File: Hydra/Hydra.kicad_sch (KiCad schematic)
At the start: 116 parts, among them J1 USB_C_Receptacle_USB2.0, SW1 SW_Push, U1 USBLC6-2SC6, U2 ATmega32U4-M, Y1 16MHz

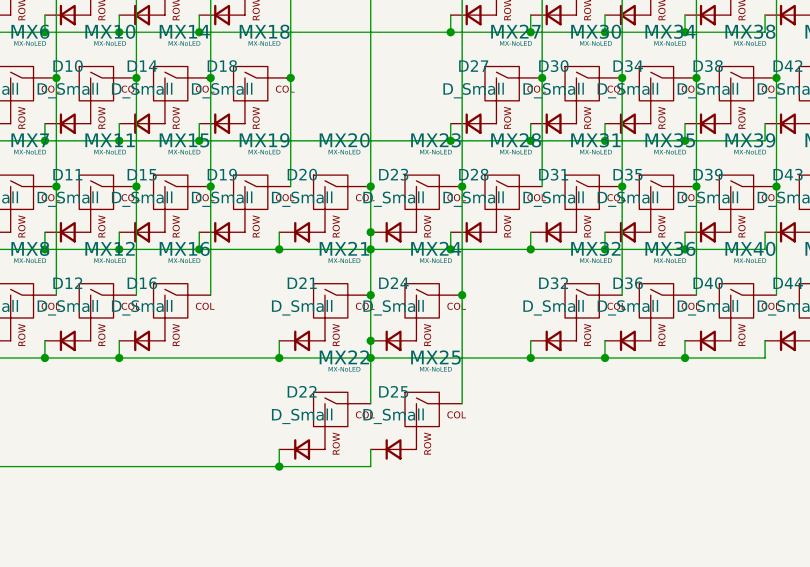
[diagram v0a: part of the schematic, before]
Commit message: Fixed Schematic
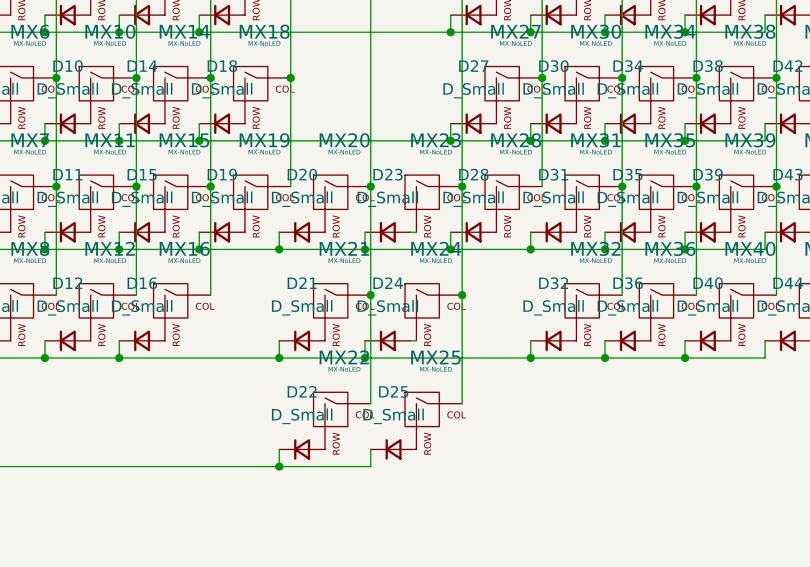
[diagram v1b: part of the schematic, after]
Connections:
- net COL5: no longer D11.1 (K), D12.1 (K), D15.1 (K), D16.1 (K), D19.1 (K), D20.1 (K), D21.1 (K), D23.1 (K), D24.1 (K), D28.1 (K), D3.1 (K), D31.1 (K), D32.1 (K), D35.1 (K), D36.1 (K), D39.1 (K), D4.1 (K), D40.1 (K), D43.1 (K), D44.1 (K), D7.1 (K), D8.1 (K)
- new net ROW2: D11.1 (K), D15.1 (K), D19.1 (K), D20.1 (K), D23.1 (K), D28.1 (K), D3.1 (K), D31.1 (K), D35.1 (K), D39.1 (K), D43.1 (K), D7.1 (K)
- new net ROW3: D12.1 (K), D16.1 (K), D21.1 (K), D24.1 (K), D32.1 (K), D36.1 (K), D4.1 (K), D40.1 (K), D44.1 (K), D8.1 (K)
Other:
- moved on the sheet: D23, D24
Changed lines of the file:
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@@
   (junction (at 68.58 111.125) (diameter 0) (color 0 0 0 0)
   )
-  (junction (at 91.44 64.135) (diameter 0) (color 0 0 0 0)
-  )
   (junction (at 191.135 41.275) (diameter 0) (color 0 0 0 0)
   )
@@
   (junction (at 117.475 52.07) (diameter 0) (color 0 0 0 0)
   )
+  (junction (at 91.44 57.15) (diameter 0) (color 0 0 0 0)
+  )
   (junction (at 144.145 142.24) (diameter 0) (color 0 0 0 0)
   )
+  (junction (at 91.44 69.215) (diameter 0) (color 0 0 0 0)
+  )
   (junction (at 46.355 40.005) (diameter 0) (color 0 0 0 0)
   )
-  (junction (at 91.44 69.215) (diameter 0) (color 0 0 0 0)
-  )
   (junction (at 82.55 45.085) (diameter 0) (color 0 0 0 0)
   )
@@
   (junction (at 55.245 40.005) (diameter 0) (color 0 0 0 0)
   )
-  (junction (at 91.44 57.15) (diameter 0) (color 0 0 0 0)
-  )
   (junction (at 109.22 64.135) (diameter 0) (color 0 0 0 0)
   )
@@
   (junction (at 217.805 31.115) (diameter 0) (color 0 0 0 0)
   )
-  (junction (at 91.44 74.295) (diameter 0) (color 0 0 0 0)
+  (junction (at 90.805 76.2) (diameter 0) (color 0 0 0 0)
   )
   (junction (at 81.28 76.2) (diameter 0) (color 0 0 0 0)
@@
   (junction (at 101.6 57.15) (diameter 0) (color 0 0 0 0)
   )
-  (junction (at 91.44 62.23) (diameter 0) (color 0 0 0 0)
-  )
   (junction (at 126.365 64.135) (diameter 0) (color 0 0 0 0)
   )
-  (junction (at 91.44 76.2) (diameter 0) (color 0 0 0 0)
-  )
   (junction (at 65.405 45.085) (diameter 0) (color 0 0 0 0)
   )
@@
   )
   (junction (at 63.5 52.07) (diameter 0) (color 0 0 0 0)
+  )
+  (junction (at 90.805 64.135) (diameter 0) (color 0 0 0 0)
   )
   (junction (at 55.245 64.135) (diameter 0) (color 0 0 0 0)
@@
     (stroke (width 0) (type default) (color 0 0 0 0))
   )
-  (wire (pts (xy 91.44 74.295) (xy 91.44 76.2))
+  (wire (pts (xy 91.44 69.215) (xy 91.44 81.28))
     (stroke (width 0) (type default) (color 0 0 0 0))
   )
@@
     (stroke (width 0) (type default) (color 0 0 0 0))
   )
-  (wire (pts (xy 91.44 62.23) (xy 91.44 64.135))
-    (stroke (width 0) (type default) (color 0 0 0 0))
-  )
   (wire (pts (xy 123.825 142.24) (xy 137.16 142.24))
     (stroke (width 0) (type default) (color 0 0 0 0))
@@
     (stroke (width 0) (type default) (color 0 0 0 0))
   )
-  (wire (pts (xy 91.44 76.2) (xy 81.28 76.2))
-    (stroke (width 0) (type default) (color 0 0 0 0))
-  )
   (wire (pts (xy 60.325 113.665) (xy 63.5 113.665))
     (stroke (width 0) (type default) (color 0 0 0 0))
@@
     (stroke (width 0) (type default) (color 0 0 0 0))
   )
+  (wire (pts (xy 91.44 57.15) (xy 91.44 69.215))
+    (stroke (width 0) (type default) (color 0 0 0 0))
+  )
   (wire (pts (xy 82.55 45.085) (xy 82.55 57.15))
     (stroke (width 0) (type default) (color 0 0 0 0))
@@
     (stroke (width 0) (type default) (color 0 0 0 0))
   )
+  (wire (pts (xy 90.805 62.23) (xy 90.805 64.135))
+    (stroke (width 0) (type default) (color 0 0 0 0))
+  )
   (wire (pts (xy 37.465 50.165) (xy 37.465 52.07))
     (stroke (width 0) (type default) (color 0 0 0 0))
@@
     (stroke (width 0) (type default) (color 0 0 0 0))
   )
-  (wire (pts (xy 91.44 57.15) (xy 91.44 62.23))
-    (stroke (width 0) (type default) (color 0 0 0 0))
-  )
   (wire (pts (xy 101.6 22.86) (xy 101.6 57.15))
     (stroke (width 0) (type default) (color 0 0 0 0))
@@
     (stroke (width 0) (type default) (color 0 0 0 0))
   )
+  (wire (pts (xy 95.885 62.23) (xy 96.52 62.23))
+    (stroke (width 0) (type default) (color 0 0 0 0))
+  )
   (wire (pts (xy 37.465 52.07) (xy 36.83 52.07))
     (stroke (width 0) (type default) (color 0 0 0 0))
   )
-  (wire (pts (xy 109.22 76.2) (xy 91.44 76.2))
+  (wire (pts (xy 81.28 76.2) (xy 90.805 76.2))
     (stroke (width 0) (type default) (color 0 0 0 0))
   )
@@
     (stroke (width 0) (type default) (color 0 0 0 0))
   )
-  (wire (pts (xy 91.44 76.2) (xy 91.44 81.28))
-    (stroke (width 0) (type default) (color 0 0 0 0))
-  )
   (wire (pts (xy 144.145 137.16) (xy 150.495 137.16))
     (stroke (width 0) (type default) (color 0 0 0 0))
@@
     (stroke (width 0) (type default) (color 0 0 0 0))
   )
+  (wire (pts (xy 90.805 76.2) (xy 109.22 76.2))
+    (stroke (width 0) (type default) (color 0 0 0 0))
+  )
   (wire (pts (xy 65.405 45.085) (xy 65.405 57.15))
     (stroke (width 0) (type default) (color 0 0 0 0))
@@
     (stroke (width 0) (type default) (color 0 0 0 0))
   )
-  (wire (pts (xy 91.44 64.135) (xy 81.28 64.135))
-    (stroke (width 0) (type default) (color 0 0 0 0))
-  )
   (wire (pts (xy 252.095 84.455) (xy 256.54 84.455))
     (stroke (width 0) (type default) (color 0 0 0 0))
@@
     (stroke (width 0) (type default) (color 0 0 0 0))
   )
+  (wire (pts (xy 95.885 74.295) (xy 96.52 74.295))
+    (stroke (width 0) (type default) (color 0 0 0 0))
+  )
   (wire (pts (xy 127.635 45.085) (xy 127.635 57.15))
     (stroke (width 0) (type default) (color 0 0 0 0))
@@
     (stroke (width 0) (type default) (color 0 0 0 0))
   )
-  (wire (pts (xy 100.33 64.135) (xy 91.44 64.135))
+  (wire (pts (xy 81.28 64.135) (xy 90.805 64.135))
     (stroke (width 0) (type default) (color 0 0 0 0))
   )
@@
     (stroke (width 0) (type default) (color 0 0 0 0))
   )
-  (wire (pts (xy 91.44 69.215) (xy 91.44 74.295))
-    (stroke (width 0) (type default) (color 0 0 0 0))
-  )
   (wire (pts (xy 36.83 76.2) (xy 36.83 74.295))
     (stroke (width 0) (type default) (color 0 0 0 0))
@@
     (stroke (width 0) (type default) (color 0 0 0 0))
   )
+  (wire (pts (xy 90.805 64.135) (xy 100.33 64.135))
+    (stroke (width 0) (type default) (color 0 0 0 0))
+  )
   (wire (pts (xy 203.2 31.115) (xy 205.74 31.115))
     (stroke (width 0) (type default) (color 0 0 0 0))
@@
     (stroke (width 0) (type default) (color 0 0 0 0))
   )
+  (wire (pts (xy 90.805 74.295) (xy 90.805 76.2))
+    (stroke (width 0) (type default) (color 0 0 0 0))
+  )
   (wire (pts (xy 100.33 38.1) (xy 100.33 40.005))
     (stroke (width 0) (type default) (color 0 0 0 0))
@@
   )
   (wire (pts (xy 135.255 64.135) (xy 126.365 64.135))
-    (stroke (width 0) (type default) (color 0 0 0 0))
-  )
-  (wire (pts (xy 91.44 64.135) (xy 91.44 69.215))
     (stroke (width 0) (type default) (color 0 0 0 0))
   )
@@
     (pin "1")
   )
-  (symbol (lib_id "Device:D_Small") (at 93.98 62.23 0) (unit 1)
-    (in_bom yes) (on_board yes) (fields_autoplaced)
-    (property "Reference" "D23" (id 0) (at 93.98 55.88 0))
-    (property "Value" "D_Small" (id 1) (at 93.98 58.42 0))
-    (property "Footprint" "Diode_SMD:D_SOD-123" (id 2) (at 93.98 62.23 90)
-      (effects (font (size 1.27 1.27)) hide)
-    )
-    (property "Datasheet" "~" (id 3) (at 93.98 62.23 90)
+  (symbol (lib_id "Device:D_Small") (at 93.345 62.23 0) (unit 1)
+    (in_bom yes) (on_board yes) (fields_autoplaced)
+    (property "Reference" "D23" (id 0) (at 93.345 55.88 0))
+    (property "Value" "D_Small" (id 1) (at 93.345 58.42 0))
+    (property "Footprint" "Diode_SMD:D_SOD-123" (id 2) (at 93.345 62.23 90)
+      (effects (font (size 1.27 1.27)) hide)
+    )
+    (property "Datasheet" "~" (id 3) (at 93.345 62.23 90)
       (effects (font (size 1.27 1.27)) hide)
     )
@@
     (pin "1")
   )
-  (symbol (lib_id "Device:D_Small") (at 93.98 74.295 0) (unit 1)
-    (in_bom yes) (on_board yes) (fields_autoplaced)
-    (property "Reference" "D24" (id 0) (at 93.98 67.945 0))
-    (property "Value" "D_Small" (id 1) (at 93.98 70.485 0))
-    (property "Footprint" "Diode_SMD:D_SOD-123" (id 2) (at 93.98 74.295 90)
-      (effects (font (size 1.27 1.27)) hide)
-    )
-    (property "Datasheet" "~" (id 3) (at 93.98 74.295 90)
-      (effects (font (size 1.27 1.27)) hide)
-    )
+  (symbol (lib_id "Device:D_Small") (at 93.345 74.295 0) (unit 1)
+    (in_bom yes) (on_board yes) (fields_autoplaced)
+    (property "Reference" "D24" (id 0) (at 93.345 67.945 0))
+    (property "Value" "D_Small" (id 1) (at 93.345 70.485 0))
+    (property "Footprint" "Diode_SMD:D_SOD-123" (id 2) (at 93.345 74.295 90)
+      (effects (font (size 1.27 1.27)) hide)
+    )
+    (property "Datasheet" "~" (id 3) (at 93.345 74.295 90)
+      (effects (font (size 1.27 1.27)) hide)
+    )
